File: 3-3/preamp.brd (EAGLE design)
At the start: 19.4 x 24 mm, 23 parts, among them Q1 SST201, Q2 SST201, Q3 SST201

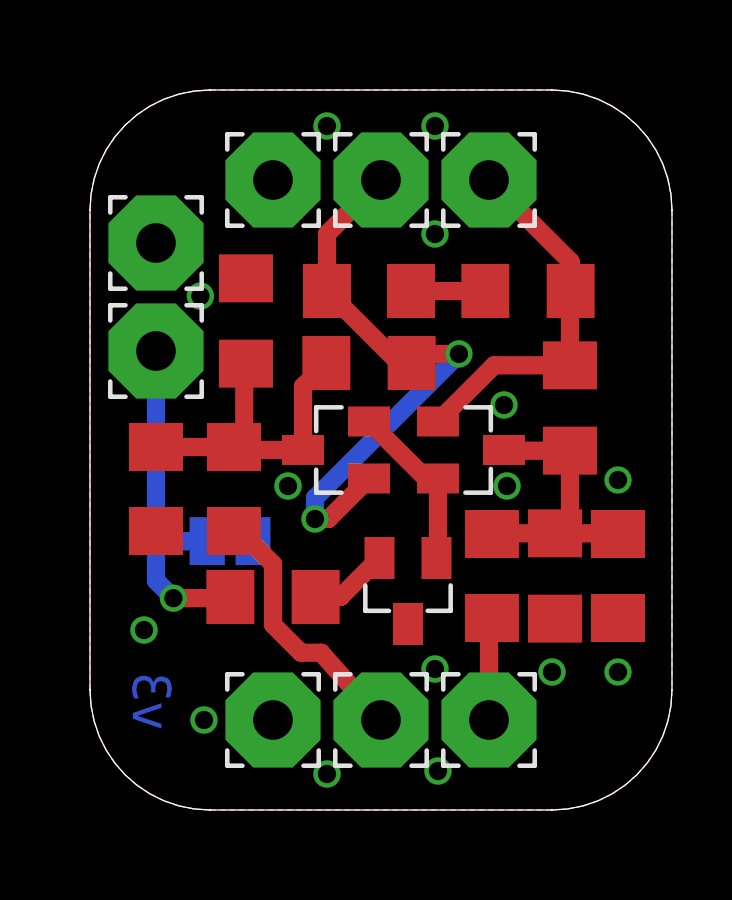
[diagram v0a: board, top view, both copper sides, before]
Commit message: Base 3-3 after 1-1 after building 2-2
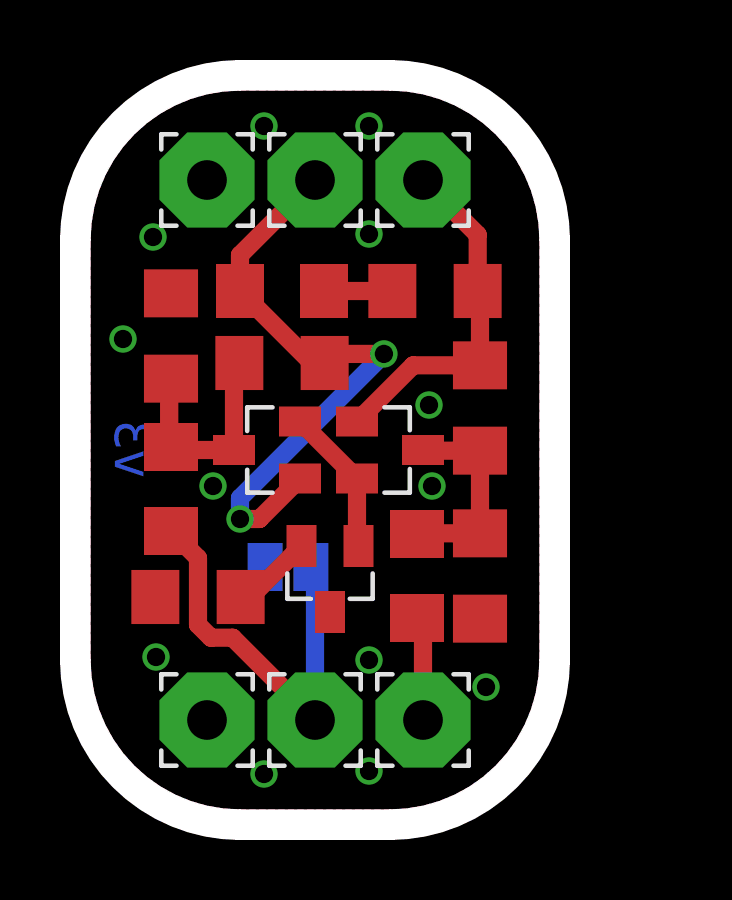
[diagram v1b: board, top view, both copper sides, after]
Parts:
- removed C4, C5: DNP, rcl:C1206
- removed POT1, POT2: (no value), wirepad:3,17/1,3
- R3: value 500 -> 510R
- moved R4 3.10 mm to (11.5, 17.3)
- moved R6 3.00 mm to (13.0, 13.4)
- moved C1 2.90 mm to (6.40, 17.3)
- moved R5 2.90 mm to (6.40, 14.9)
- moved Q2 2.70 mm to (10.0, 12.0)
- moved Q3 2.63 mm to (8.00, 7.70)
- moved R1 2.55 mm to (2.70, 15.8)
- moved C3 2.50 mm to (10.9, 7.80)
- moved R2 2.50 mm to (13.0, 7.80)
- moved R3 2.50 mm to (3.60, 7.10)
- moved Q1 2.30 mm to (5.90, 12.0)
- moved PZ-2 2.20 mm to (11.1, 3.00)
- moved XLR3 2.20 mm to (11.1, 21.0)
- moved PZ-GND 2.20 mm to (3.90, 3.00)
- moved XLR1 2.20 mm to (3.90, 21.0)
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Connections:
- removed net N$2: POT1.1, R3.1, SJ1.2
- net GND: now also R3.1; no longer C4.1, C5.1, POT2.1
- net N$3: no longer C4.2
- net N$7: no longer C5.2
- net PZ-1: now also SJ1.2
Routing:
- net N$2: track 12.1 -> 0.00 mm, vias 1 -> 0
- net PZ-1: track 8.74 -> 13.9 mm
- net N$3: track 12.2 -> 7.46 mm
- net N$7: track 9.40 -> 6.79 mm
- net XLR-2: track 19.8 -> 20.8 mm
- net N$1: track 5.76 -> 4.96 mm
- net XLR3: track 12.5 -> 11.8 mm
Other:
- board size 19.4 x 24 mm -> 16 x 25 mm
- board text added: "Piezo Pre-amp 181205"
- board text removed: "Piezo Pre-amp 181204 v3"
